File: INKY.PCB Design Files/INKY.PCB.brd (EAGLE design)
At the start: 55.8 x 40.9 mm, 34 parts, among them J1-PROG RJ45-8MOLEX_0955406886, J2 RJ45-8MOLEX_0955406886, U1 MC9S08SH8CTG, U3 RS485SOIC

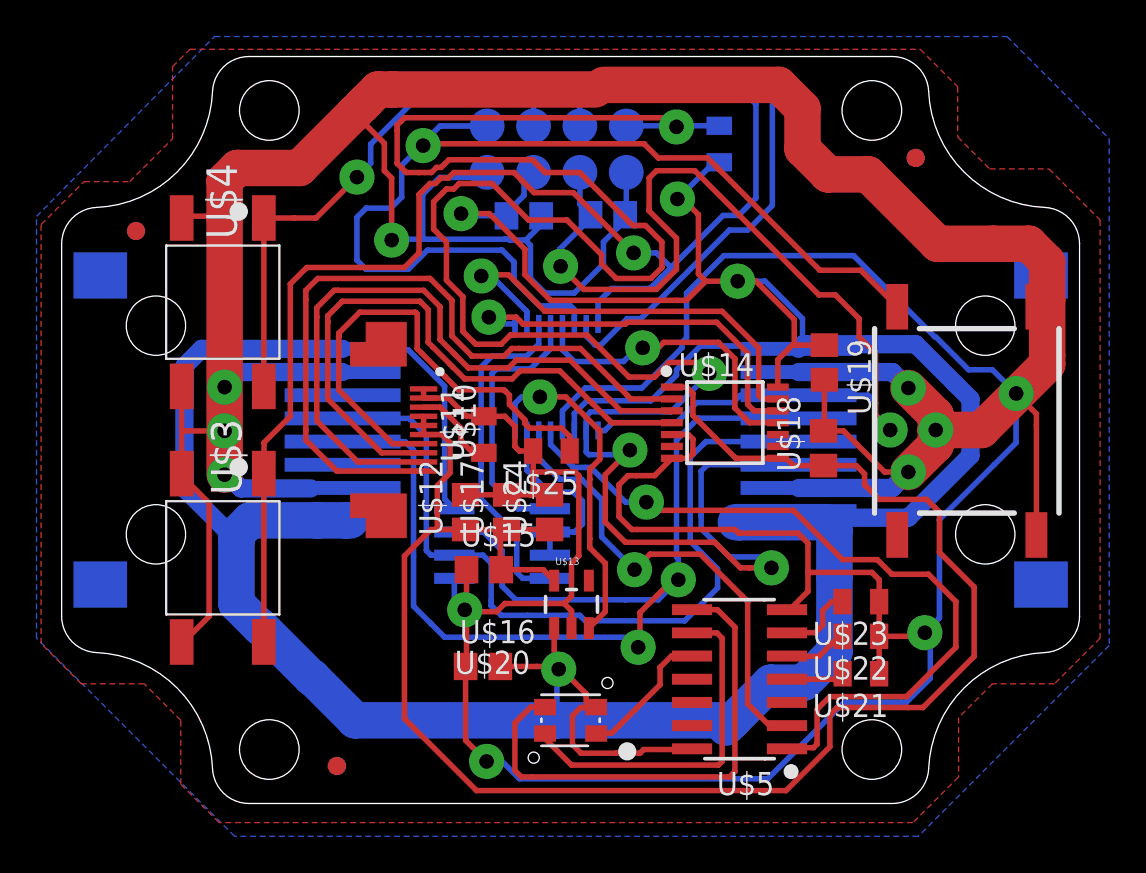
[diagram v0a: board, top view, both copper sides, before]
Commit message: Inky 0.2
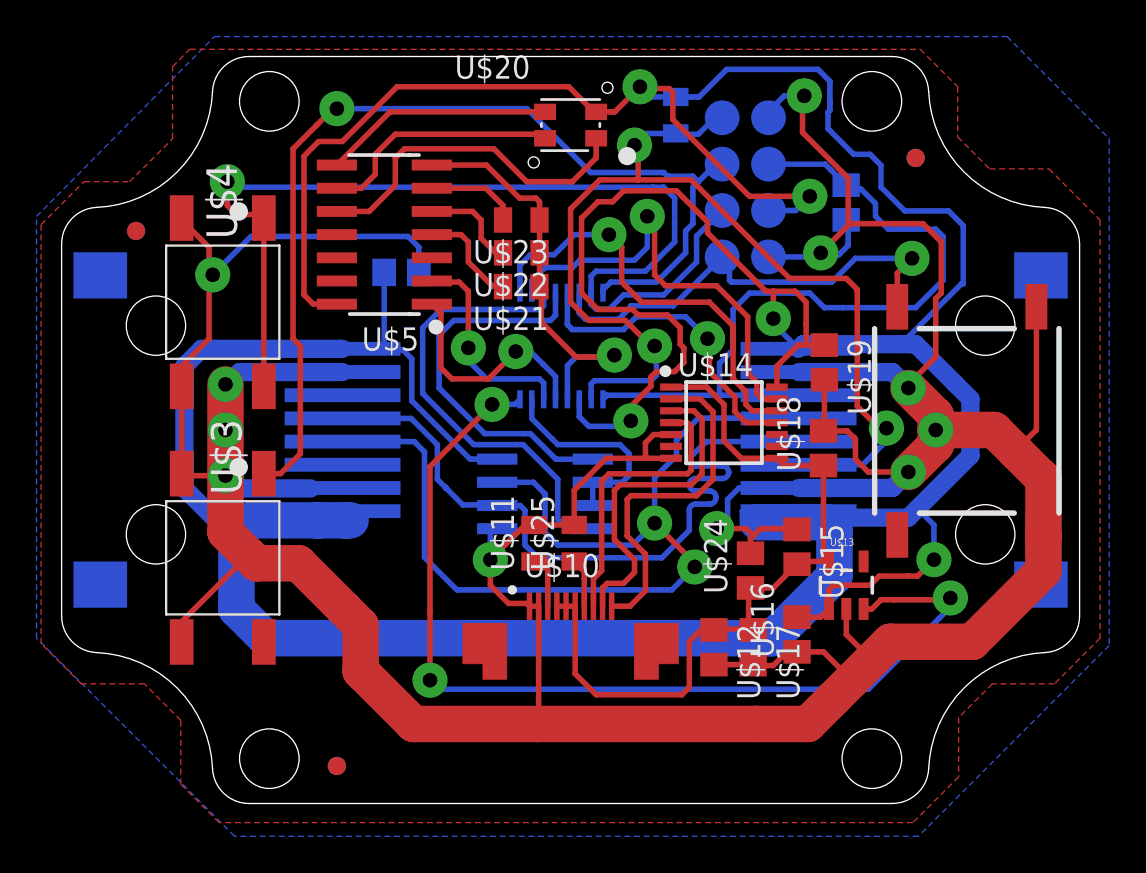
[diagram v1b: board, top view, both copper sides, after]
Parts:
- U$11, U$25: value (none) -> 10K
- moved U$20 32.6 mm to (0.00, 16.7)
- moved U$5 31.2 mm to (-10.2, 10.7)
- moved U$21 28.2 mm to (-2.70, 7.85)
- moved U$22 28.1 mm to (-2.70, 9.70)
- moved U$23 28.0 mm to (-2.70, 11.5)
- moved U$16 17.3 mm to (12.4, -11.2), turned to 90 degrees
- moved U$15 17.2 mm to (12.4, -6.40), turned to 270 degrees
- moved U$12 15.5 mm to (7.85, -11.9), turned to 270 degrees
- moved U$17 15.4 mm to (10.0, -11.9), turned to 270 degrees
- moved U$13 15.1 mm to (15.1, -8.50)
- moved U$10 13.9 mm to (0.00, -10.6), turned to 0 degrees
- moved C2 13.1 mm to (15.1, 12.5), turned to 90 degrees
- moved U$24 11.5 mm to (9.85, -7.70)
- moved C1 7.38 mm to (-9.26, 8.63)
- moved U$11 6.55 mm to (-2.00, -6.20)
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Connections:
- net INC_DOWN: no longer U$3.2
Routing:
- net GND: track 358.6 -> 283.5 mm, vias 11 -> 12
- net BDM: track 120.5 -> 57.8 mm, vias 4 -> 3
- net GMD: track 94.8 -> 42.5 mm
- net +5V: track 208.9 -> 259.3 mm, vias 4 -> 5
- net N$1: track 18.9 -> 54.2 mm, vias 1 -> 3
- net ACK: track 57.9 -> 25.7 mm
- net N$6: track 41.7 -> 12.7 mm
- net N$33: track 27.3 -> 2.68 mm
- net N$2: track 39.9 -> 19.1 mm
- net INC_DOWN: track 76.5 -> 56.1 mm
- net N$3: track 37.0 -> 18.1 mm
- net N$4: track 34.4 -> 15.8 mm
- net RST: track 58.9 -> 42.6 mm, vias 2 -> 0
- net N$9: track 27.6 -> 12.6 mm
- net N$5: track 26.4 -> 11.6 mm
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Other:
- board text added: "INKY.PCB.v1.0P2"
- board text removed: "POSCON.PCB.v1.2"
